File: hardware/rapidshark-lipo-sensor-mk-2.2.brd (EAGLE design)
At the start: 35.6 x 20.3 mm, 13 parts, among them IC1 Tiny84, Q1 2N7000, Q2 2N7000, Q3 2N7000

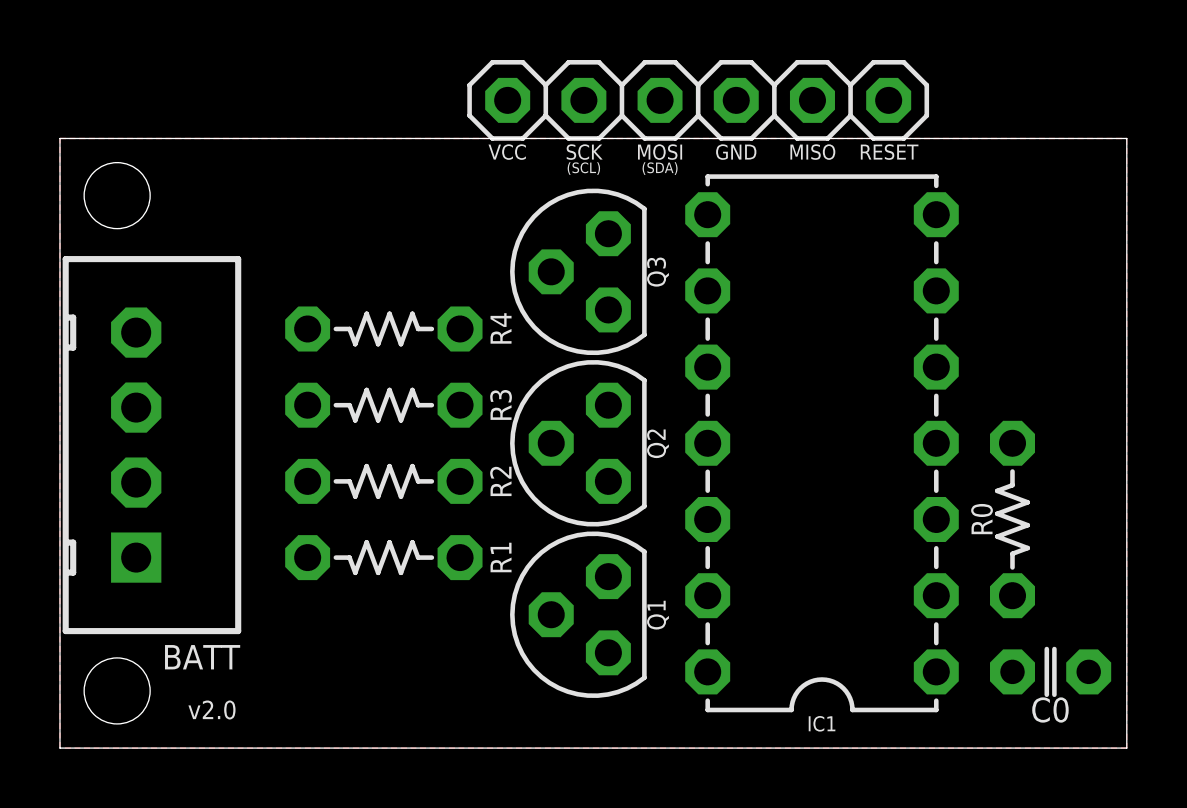
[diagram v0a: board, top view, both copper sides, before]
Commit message: lipo voltage testing boards
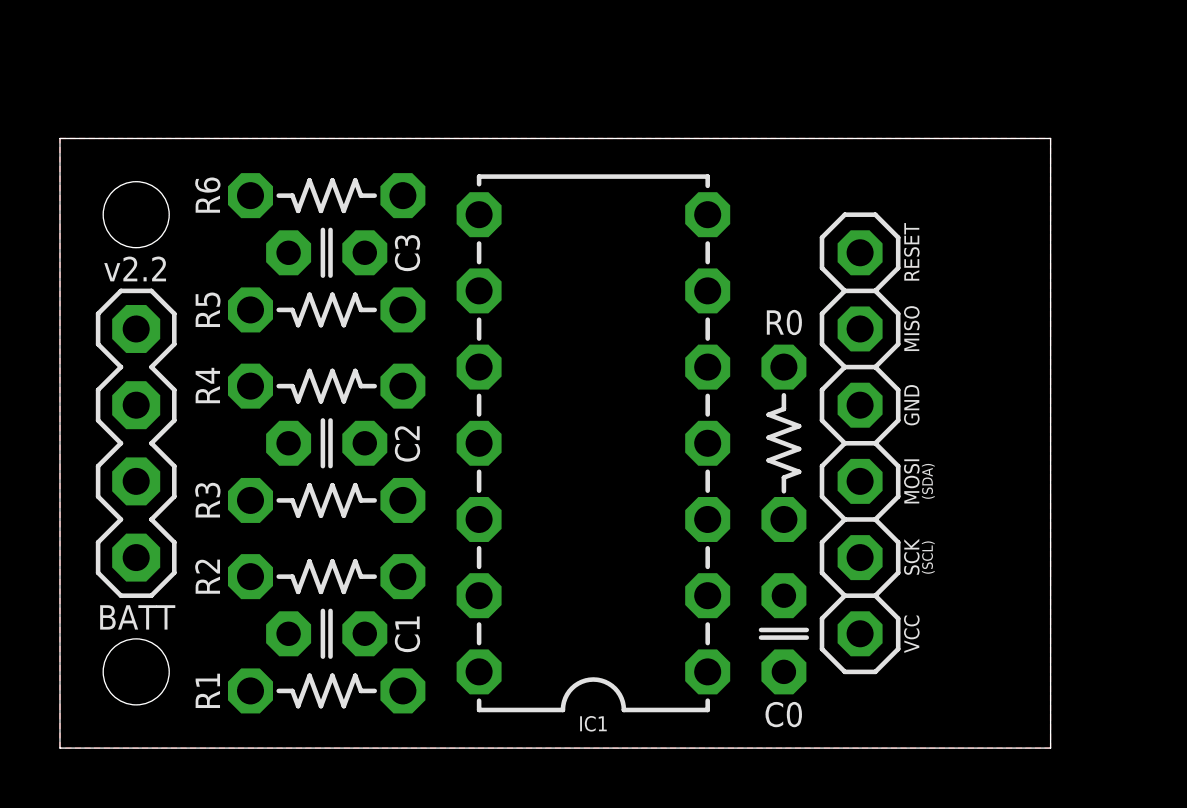
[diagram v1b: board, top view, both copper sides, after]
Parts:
- removed Q1, Q2, Q3: 2N7000, a_parts:TO-92
- added C1, C2, C3: 100n, A_butts:C025-024X044
- added R5, R6: 10k, A_butts:RESISTOR-AXIAL-PTH-5.08MM
- BATT: value M04JST_XH_VERT -> M04PTH; device a_parts:JST-4-XH-VERT-TH -> a_parts:1X04-PTH-VERT
- moved AVRISP 12.6 mm to (26.7, 10.2), turned to 90 degrees
- moved C0 8.98 mm to (24.1, 3.81), turned to 90 degrees
- moved R0 8.03 mm to (24.1, 10.2)
- moved IC1 7.62 mm to (17.8, 10.2)
- moved R1 4.84 mm to (8.89, 1.91), turned to 0 degrees
- moved R2 3.70 mm to (8.89, 5.71)
- moved R3 3.70 mm to (8.89, 8.26), turned to 0 degrees
- moved R4 2.69 mm to (8.89, 12.1)
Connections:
- removed net EN1: IC1.2, Q1.2
- removed net EN2: IC1.3, Q2.2
- removed net EN3: IC1.5, Q3.2
- removed net N$3: Q3.3, R4.P$1
- net BATT-: now also C1.2, R1.P$1; no longer R1.P$2
- net CELL1+: now also C2.2, R3.P$1
- net CELL2+: now also C3.2, R4.P$2, R5.P$1; no longer R3.P$2
- net CELL3+: now also R6.P$2; no longer R4.P$2
- net VDIV1: now also C1.1, R1.P$2, R2.P$1; no longer Q1.1, R1.P$1
- net VDIV2: now also C2.1, R3.P$2, R4.P$1; no longer Q1.3, Q2.1, R2.P$1
- net VDIV3: now also C3.1, R5.P$2, R6.P$1; no longer Q2.3, Q3.1, R3.P$1
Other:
- board size 35.6 x 20.3 mm -> 33 x 20.3 mm
